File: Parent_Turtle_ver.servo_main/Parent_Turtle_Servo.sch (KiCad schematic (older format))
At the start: 45 parts, among them P1 CONN_02X15, P10 WRITING, P11 A/D, P12 5V_in, P2 CONN_02X15, P3 CAN, P4 CAN, P5 PWM, P6 SERIAL0, P7 SERIAL1, P8 WRITING_IN, P9 CAN_JP, Q1 NPN, SW1 SW_PUSH, SW2 SW_PUSH, U1 MAX3051

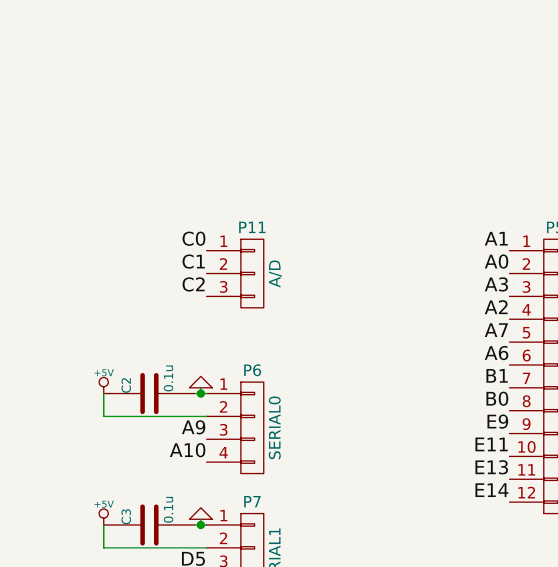
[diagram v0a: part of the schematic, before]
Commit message: バージョンを上げた
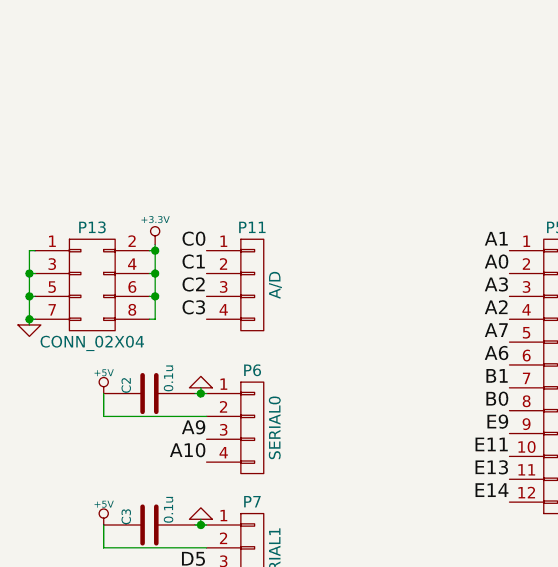
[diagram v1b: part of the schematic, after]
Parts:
- removed P11: A/D, Pin_Headers:Pin_Header_Straight_1x03, symbol CONN_01X03
- added P11: A/D, Pin_Headers:Pin_Header_Straight_1x04, symbol CONN_01X04
- added P13: CONN_02X04, Pin_Headers:Pin_Header_Straight_2x04, symbol CONN_02X04
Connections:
- net +3.3V: now also P13.2 (P2), P13.4 (P4), P13.6 (P6), P13.8 (P8)
- net C0: now also P11.1 (P1)
- net C1: now also P11.2 (P2)
- net C2: now also P11.3 (P3)
- net C3: now also P11.4 (P4)
- net GND: now also P13.1 (P1), P13.3 (P3), P13.5 (P5), P13.7 (P7)
